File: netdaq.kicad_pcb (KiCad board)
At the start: 2 copper layers, 127.5 x 83 mm, 288 parts, among them J1 RJ45, J3 Conn_01x06_Pin, J4 Micro_SD_Card_Det2, U1 PIC32CK1025GC01100-I/4SB, U10 TLA2518IRTER, U11 TLA2518IRTER, U2 LAN8720A-CP, U5 MP6004GQ-P, U6 PD70100ILD-TR, U7 TPS62A01PDDCR, U8 TLA2518IRTER, U9 TLA2518IRTER

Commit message: did stuff
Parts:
- moved TR1 159.4 mm to (170.0, 75.3)
- moved C114 158.9 mm to (105.1, 97.5), turned to -90 degrees
- moved J1 157.8 mm to (174.3, 61.1)
- moved C113 156.6 mm to (107.6, 98.3), turned to -90 degrees
- moved C6 155.7 mm to (184.5, 112.0), turned to 180 degrees
- moved R84 153.1 mm to (110.1, 97.5), turned to -90 degrees
- moved R85 150.7 mm to (112.1, 97.5), turned to -90 degrees
- moved R86 148.4 mm to (114.0, 97.5), turned to -90 degrees
- moved C4 147.1 mm to (186.4, 106.0), turned to 0 degrees
- moved C13 146.5 mm to (180.8, 111.2), turned to 0 degrees
- moved R87 146.2 mm to (116.0, 97.5), turned to -90 degrees
- moved R88 143.9 mm to (118.0, 97.5), turned to -90 degrees
- moved R89 141.7 mm to (120.0, 97.5), turned to -90 degrees
- moved R90 139.5 mm to (122.0, 97.5), turned to -90 degrees
- moved C5 138.4 mm to (183.5, 105.9), turned to 0 degrees
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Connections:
- J2 pad 1: /DAQ Connector/EXT_ADC1 -> unconnected-(J2-Pin_1-Pad1)
- J2 pad 10: /DAQ Connector/EXT_ADC10 -> /DAQ Connector/EXT_ADC6
- J2 pad 11: /DAQ Connector/EXT_ADC11 -> /DAQ Connector/EXT_ADC7
- J2 pad 12: /DAQ Connector/EXT_ADC12 -> /DAQ Connector/EXT_ADC8
- J2 pad 13: /DAQ Connector/EXT_ADC13 -> /DAQ Connector/EXT_ADC9
- J2 pad 14: /DAQ Connector/EXT_ADC14 -> /DAQ Connector/EXT_ADC10
- J2 pad 15: /DAQ Connector/EXT_ADC15 -> /DAQ Connector/EXT_ADC11
- J2 pad 16: /DAQ Connector/EXT_ADC16 -> /DAQ Connector/EXT_ADC12
- J2 pad 17: /DAQ Connector/EXT_ADC17 -> /DAQ Connector/EXT_ADC13
- J2 pad 18: /DAQ Connector/EXT_ADC18 -> /DAQ Connector/EXT_ADC14
- J2 pad 19: /DAQ Connector/EXT_ADC19 -> /DAQ Connector/EXT_ADC15
- J2 pad 2: /DAQ Connector/EXT_ADC2 -> unconnected-(J2-Pin_2-Pad2)
- J2 pad 20: /DAQ Connector/EXT_ADC20 -> /DAQ Connector/EXT_ADC16
- J2 pad 21: /DAQ Connector/EXT_ADC21 -> /DAQ Connector/EXT_ADC17
- J2 pad 22: /DAQ Connector/EXT_ADC22 -> /DAQ Connector/EXT_ADC18
- J2 pad 23: /DAQ Connector/EXT_ADC23 -> /DAQ Connector/EXT_ADC19
- J2 pad 24: /DAQ Connector/EXT_ADC24 -> /DAQ Connector/EXT_ADC20
- J2 pad 25: /DAQ Connector/EXT_ADC25 -> /DAQ Connector/EXT_ADC21
- J2 pad 26: /DAQ Connector/EXT_ADC26 -> /DAQ Connector/EXT_ADC22
- J2 pad 27: /DAQ Connector/EXT_ADC27 -> /DAQ Connector/EXT_ADC23
- J2 pad 28: /DAQ Connector/EXT_ADC28 -> /DAQ Connector/EXT_ADC24
- J2 pad 29: /DAQ Connector/EXT_ADC29 -> /DAQ Connector/EXT_ADC25
- J2 pad 3: /DAQ Connector/EXT_ADC3 -> unconnected-(J2-Pin_3-Pad3)
- J2 pad 30: /DAQ Connector/EXT_ADC30 -> /DAQ Connector/EXT_ADC26
- J2 pad 31: /DAQ Connector/EXT_ADC31 -> /DAQ Connector/EXT_ADC27
- J2 pad 32: /DAQ Connector/EXT_ADC32 -> /DAQ Connector/EXT_ADC28
- J2 pad 33: unconnected-(J2-Pin_33-Pad33) -> /DAQ Connector/EXT_ADC29
- J2 pad 34: unconnected-(J2-Pin_34-Pad34) -> /DAQ Connector/EXT_ADC30
- J2 pad 35: unconnected-(J2-Pin_35-Pad35) -> /DAQ Connector/EXT_ADC31
- J2 pad 36: unconnected-(J2-Pin_36-Pad36) -> /DAQ Connector/EXT_ADC32
- J2 pad 37: unconnected-(J2-Pin_37-Pad37) -> GND
- J2 pad 38: unconnected-(J2-Pin_38-Pad38) -> GND
- J2 pad 4: /DAQ Connector/EXT_ADC4 -> unconnected-(J2-Pin_4-Pad4)
- J2 pad 5: /DAQ Connector/EXT_ADC5 -> /DAQ Connector/EXT_ADC1
- J2 pad 6: /DAQ Connector/EXT_ADC6 -> /DAQ Connector/EXT_ADC2
- J2 pad 7: /DAQ Connector/EXT_ADC7 -> /DAQ Connector/EXT_ADC3
- J2 pad 8: /DAQ Connector/EXT_ADC8 -> /DAQ Connector/EXT_ADC4
- J2 pad 9: /DAQ Connector/EXT_ADC9 -> /DAQ Connector/EXT_ADC5
- U1 pad 10: /MCU_SPI5_ADC3.SCK -> /ADC2/SPI.SCK
- U1 pad 11: /MCU_SPI5_ADC3.CS# -> /ADC2/SPI.CS#
- U1 pad 16: /MCU_SPI6_ADC4.MOSI -> /MCU_SPI5_ADC3.MOSI
- U1 pad 17: /MCU_SPI6_ADC4.MISO -> /MCU_SPI5_ADC3.MISO
- U1 pad 22: /MCU_SPI6_ADC4.SCK -> /MCU_SPI5_ADC3.SCK
- U1 pad 23: /MCU_SPI6_ADC4.CS# -> /MCU_SPI5_ADC3.CS#
- U1 pad 45: /MCU_SPI3_ADC2.MOSI -> /MCU_SPI6_ADC4.MOSI
- U1 pad 46: /MCU_SPI3_ADC2.MISO -> /MCU_SPI6_ADC4.MISO
- U1 pad 47: /MCU_SPI3_ADC2.SCK -> /MCU_SPI6_ADC4.SCK
- U1 pad 48: /MCU_SPI3_ADC2.CS# -> /MCU_SPI6_ADC4.CS#
- U1 pad 8: /MCU_SPI5_ADC3.MOSI -> /ADC2/SPI.MOSI
- U1 pad 9: /MCU_SPI5_ADC3.MISO -> /ADC2/SPI.MISO
- U10 pad 11: /ADC3/SPI.CS# -> /MCU_SPI5_ADC3.CS#
- U10 pad 12: /ADC3/SPI.MISO -> /MCU_SPI5_ADC3.MISO
- U10 pad 13: /ADC3/SPI.SCK -> /MCU_SPI5_ADC3.SCK
- U10 pad 14: /ADC3/SPI.MOSI -> /MCU_SPI5_ADC3.MOSI
- U11 pad 11: /ADC4/SPI.CS# -> /MCU_SPI6_ADC4.CS#
- U11 pad 12: /ADC4/SPI.MISO -> /MCU_SPI6_ADC4.MISO
- U11 pad 13: /ADC4/SPI.SCK -> /MCU_SPI6_ADC4.SCK
- U11 pad 14: /ADC4/SPI.MOSI -> /MCU_SPI6_ADC4.MOSI
- U11 pad 15: /GPIO24 -> /GPIO25
- U8 pad 11: /ADC1/SPI.CS# -> /MCU_SPI2_ADC1.CS#
- U8 pad 12: /ADC1/SPI.MISO -> /MCU_SPI2_ADC1.MISO
- U8 pad 13: /ADC1/SPI.SCK -> /MCU_SPI2_ADC1.SCK
- U8 pad 14: /ADC1/SPI.MOSI -> /MCU_SPI2_ADC1.MOSI
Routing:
- net /ADC2/SPI.MOSI: track 0.00 -> 14.4 mm
- net /ADC2/SPI.SCK: track 0.00 -> 13.3 mm
- net /ADC2/SPI.MISO: track 0.00 -> 12.1 mm, vias 0 -> 2
- net /ADC2/SPI.CS#: track 0.00 -> 11.8 mm
- net /MCU_SPI5_ADC3.MOSI: track 0.00 -> 8.57 mm
- net /MCU_SPI5_ADC3.MISO: track 0.00 -> 8.14 mm, vias 0 -> 2
- net /MCU_SPI5_ADC3.SCK: track 0.00 -> 6.69 mm
- net /MCU_SPI5_ADC3.CS#: track 0.00 -> 6.08 mm
- net unconnected-(J2-Pin_38-Pad38): track 3.72 -> 0.00 mm
- net unconnected-(J2-Pin_36-Pad36): track 3.72 -> 0.00 mm
- net unconnected-(J2-Pin_34-Pad34): track 3.72 -> 0.00 mm
- net GND: track 1.09 -> 4.82 mm
- net unconnected-(J2-Pin_4-Pad4): track 0.00 -> 3.47 mm
- net /DAQ Connector/EXT_ADC2: track 3.86 -> 7.33 mm
- net Net-(U9-DECAP): track 0.00 -> 3.19 mm
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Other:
- board size 127.5 x 83 mm -> 131.5 x 93 mm

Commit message: stuff
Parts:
- moved C35 219.7 mm to (141.5, 79.0), turned to -90 degrees
- moved U5 218.0 mm to (179.0, 58.7)
- moved C34 213.0 mm to (148.0, 79.0), turned to -90 degrees
- moved R34 205.6 mm to (155.5, 55.5), turned to 180 degrees
- moved R33 204.4 mm to (155.5, 61.5), turned to 180 degrees
- moved R37 203.8 mm to (155.5, 64.5)
- moved R35 203.4 mm to (155.5, 66.0)
- moved R38 201.1 mm to (155.5, 54.0)
- moved R36 199.5 mm to (155.5, 58.5), turned to 180 degrees
- moved R42 199.3 mm to (155.5, 57.0)
- moved R41 198.2 mm to (155.5, 60.0)
- moved R39 196.8 mm to (155.5, 63.0)
- moved R40 196.4 mm to (155.5, 67.5)
- moved TR2 192.7 mm to (186.1, 66.0), turned to -90 degrees
- moved U3 187.0 mm to (161.5, 58.0), turned to -90 degrees
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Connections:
- net /ADC2/SPI.CS# renamed /MCU_SPI3_ADC2.CS#
- net /ADC2/SPI.MISO renamed /MCU_SPI3_ADC2.MISO
- net /ADC2/SPI.MOSI renamed /MCU_SPI3_ADC2.MOSI
- net /ADC2/SPI.SCK renamed /MCU_SPI3_ADC2.SCK
- R13 pad 2: /Ethernet PHY/RMII.REFCK -> /RMII.REFCK
- R15 pad 2: /Ethernet PHY/RMII.RXER -> /RMII.RXER
- R19 pad 2: /Ethernet PHY/RMII.RXD0 -> /RMII.RXD0
- R21 pad 2: /Ethernet PHY/RMII.RXD1 -> /RMII.RXD1
- R22 pad 2: /Ethernet PHY/RMII.CRSDV -> /RMII.CRSDV
- R23 pad 1: /Ethernet PHY/RMII.RXER -> /RMII.RXER
- U1 pad 51: /MCU/RMII.REFCK -> /RMII.REFCK
- U1 pad 60: /MCU/RMII.RXD1 -> /RMII.RXD1
- U1 pad 61: /MCU/RMII.RXD0 -> /RMII.RXD0
- U1 pad 63: /MCU/RMII.RXER -> /RMII.RXER
- U1 pad 68: /MCU/RMII.CRSDV -> /RMII.CRSDV
- U1 pad 71: /MCU/RMII.TXEN -> /RMII.TXEN
- U1 pad 72: /MCU/RMII.TXD0 -> /RMII.TXD0
- U1 pad 73: /MCU/RMII.TXD1 -> /RMII.TXD1
- U2 pad 10: /Ethernet PHY/RMII.RXER -> /RMII.RXER
- U2 pad 14: /Ethernet PHY/RMII.REFCK -> /RMII.REFCK
- U2 pad 16: /Ethernet PHY/RMII.TXEN -> /RMII.TXEN
- U2 pad 17: /Ethernet PHY/RMII.TXD0 -> /RMII.TXD0
- U2 pad 18: /Ethernet PHY/RMII.TXD1 -> /RMII.TXD1
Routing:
- net /SDMMC.SDDAT0: track 0.00 -> 30.8 mm
- net /SDMMC.SDDAT2: track 0.00 -> 21.7 mm, vias 0 -> 2
- net /Ethernet Connector/MX4-: track 0.00 -> 20.8 mm
- net /SDMMC.SDDAT3: track 0.00 -> 20.6 mm, vias 0 -> 2
- net /SDMMC.SDCMD: track 0.00 -> 20.5 mm
- net /Ethernet Connector/MX4+: track 0.00 -> 17.6 mm
- net /Ethernet Connector/MX3-: track 0.00 -> 16.6 mm
- net Net-(C36-Pad1): track 0.00 -> 16.1 mm
- net /SDMMC.SDDAT1: track 0.00 -> 16.0 mm
- net /Ethernet Connector/MX3+: track 0.00 -> 12.5 mm
- net /Ethernet Connector/CTREF2: track 0.00 -> 12.2 mm
- net /SDMMC.SDWP: track 0.00 -> 11.3 mm
- net /SDMMC.SDCK: track 0.00 -> 11.3 mm
- net /Ethernet Connector/MX2+: track 0.00 -> 9.68 mm
- net /Ethernet Connector/MX1+: track 0.00 -> 7.20 mm
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
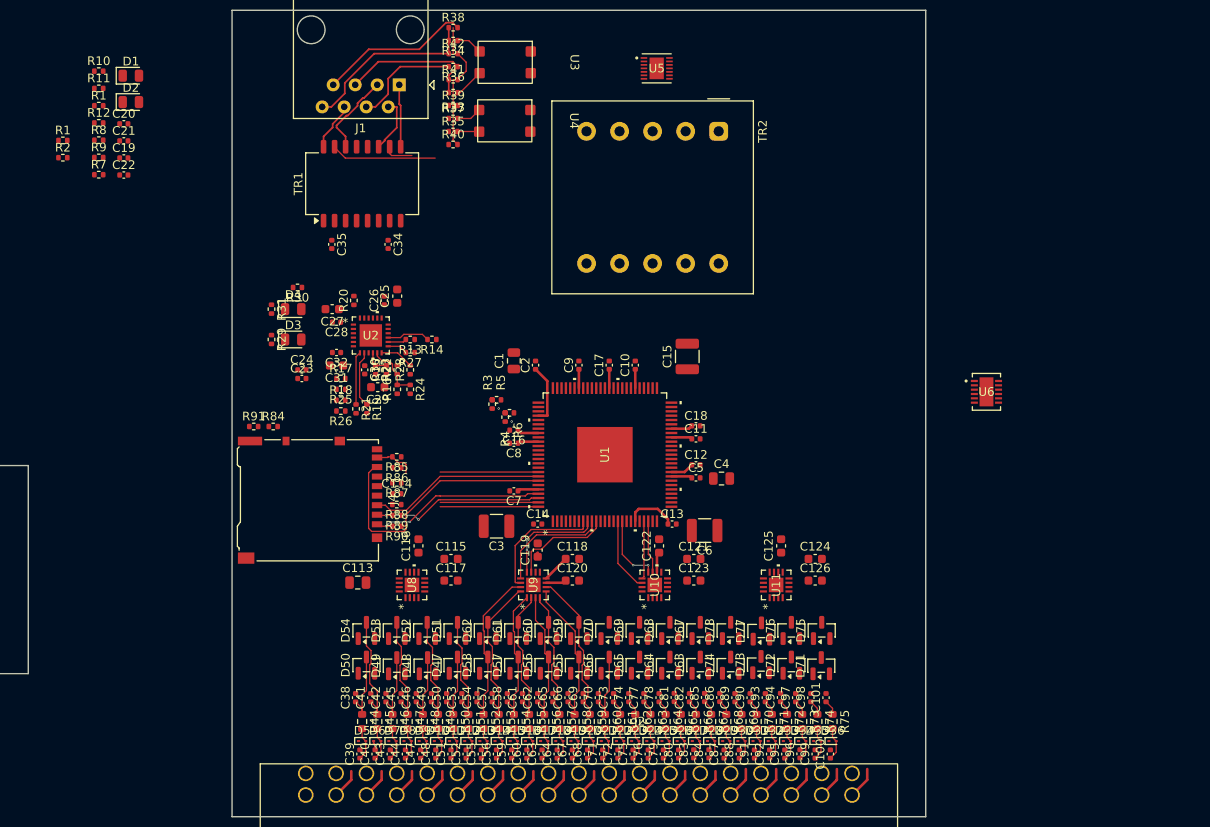
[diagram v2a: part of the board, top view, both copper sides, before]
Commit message: did some layouting
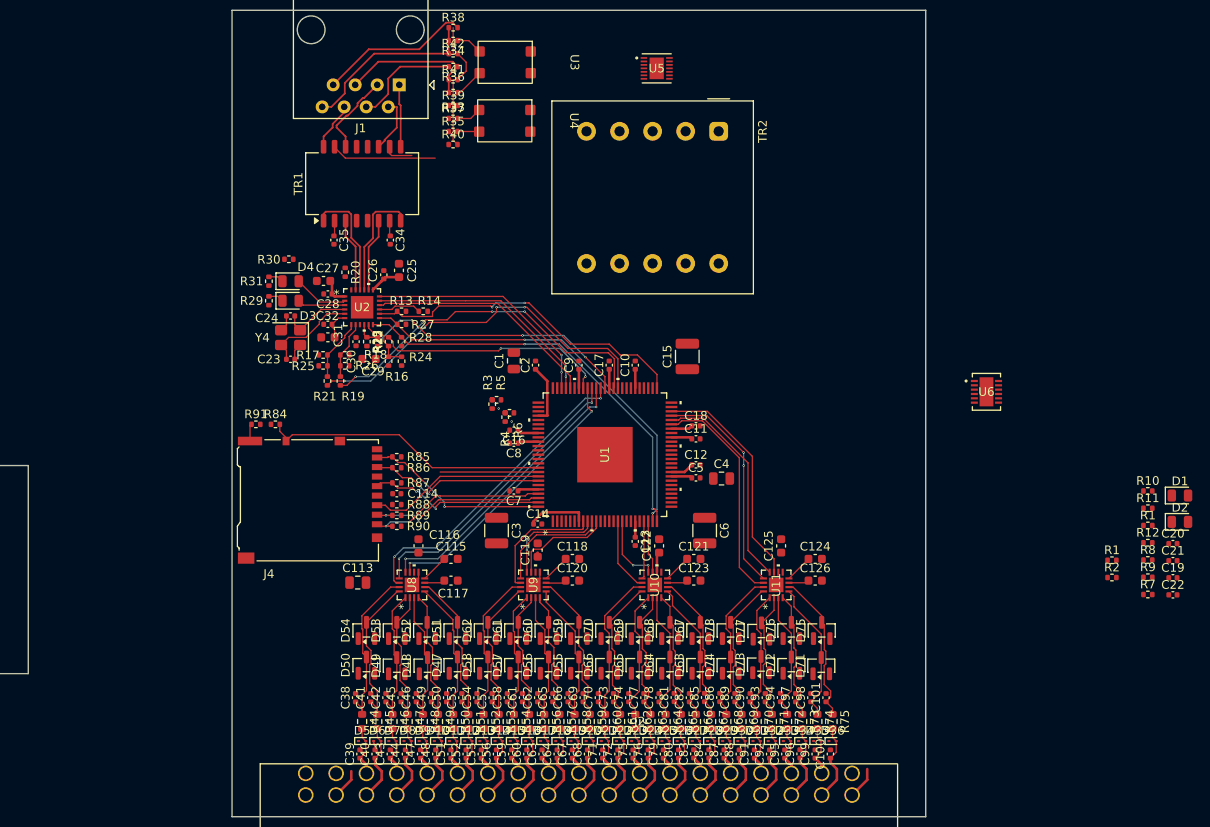
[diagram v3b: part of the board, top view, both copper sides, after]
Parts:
- added Y4: Crystal_GND24, Crystal:Crystal_SMD_Abracon_ABM8G-4Pin_3.2x2.5mm, F.Cu at (136.8, 89.8)
- moved R1 130.3 mm to (235.6, 111.4)
- moved R10 130.3 mm to (235.6, 107.4)
- moved R11 130.3 mm to (235.6, 109.4)
- moved R12 130.3 mm to (235.6, 113.4)
- moved R7 130.3 mm to (235.6, 119.4)
- moved R8 130.3 mm to (235.6, 115.4)
- moved R9 130.3 mm to (235.6, 117.4)
- moved C19 130.3 mm to (238.5, 117.4)
- moved C20 130.3 mm to (238.5, 113.5)
- moved C21 130.3 mm to (238.5, 115.5)
- moved C22 130.3 mm to (238.5, 119.4)
- moved D1 130.3 mm to (239.3, 108.0)
- moved D2 130.3 mm to (239.3, 111.0)
- moved R1 130.3 mm to (231.5, 115.4)
- moved R2 130.3 mm to (231.5, 117.4)
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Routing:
- net /SMI.MDC: track 2.33 -> 47.8 mm, vias 0 -> 2
- net /SMI.MDIO: track 3.90 -> 47.7 mm, vias 0 -> 2
- net /RMII.RXD1: track 0.00 -> 43.4 mm, vias 0 -> 4
- net /RMII.RXD0: track 0.00 -> 40.8 mm, vias 0 -> 4
- net /RMII.REFCK: track 2.15 -> 38.5 mm, vias 0 -> 2
- net /MCU_SPI2_ADC1.MOSI: track 0.00 -> 36.0 mm, vias 0 -> 2
- net /MCU_SPI2_ADC1.SCK: track 0.00 -> 33.7 mm, vias 0 -> 2
- net /SDMMC.SDCD: track 0.00 -> 33.2 mm
- net /MCU_SPI2_ADC1.MISO: track 0.00 -> 33.0 mm, vias 0 -> 2
- net /MCU_SPI2_ADC1.CS#: track 0.00 -> 32.2 mm, vias 0 -> 2
- net /RMII.RXER: track 2.83 -> 34.3 mm, vias 0 -> 4
- net /RMII.TXD1: track 0.00 -> 27.6 mm, vias 0 -> 2
- net /RMII.TXD0: track 0.00 -> 27.2 mm, vias 0 -> 2
- net /RMII.TXEN: track 0.00 -> 26.9 mm
- net /RMII.CRSDV: track 0.00 -> 26.7 mm, vias 0 -> 2
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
